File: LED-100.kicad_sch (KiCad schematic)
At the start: 101 parts, among them J2 LDA100_2_J2, J3 LDA100_2_J3, J4 LDA100_2_J4, J5 xtra, J7 Conn_01x01, J8 Conn_01x08, SW1 SW_SPDT, SW2 SW_SPST, U1 TLC5947DAP, U2 TLC5947DAP, U3 TLC5947DAP, U4 TEENSY 4.0

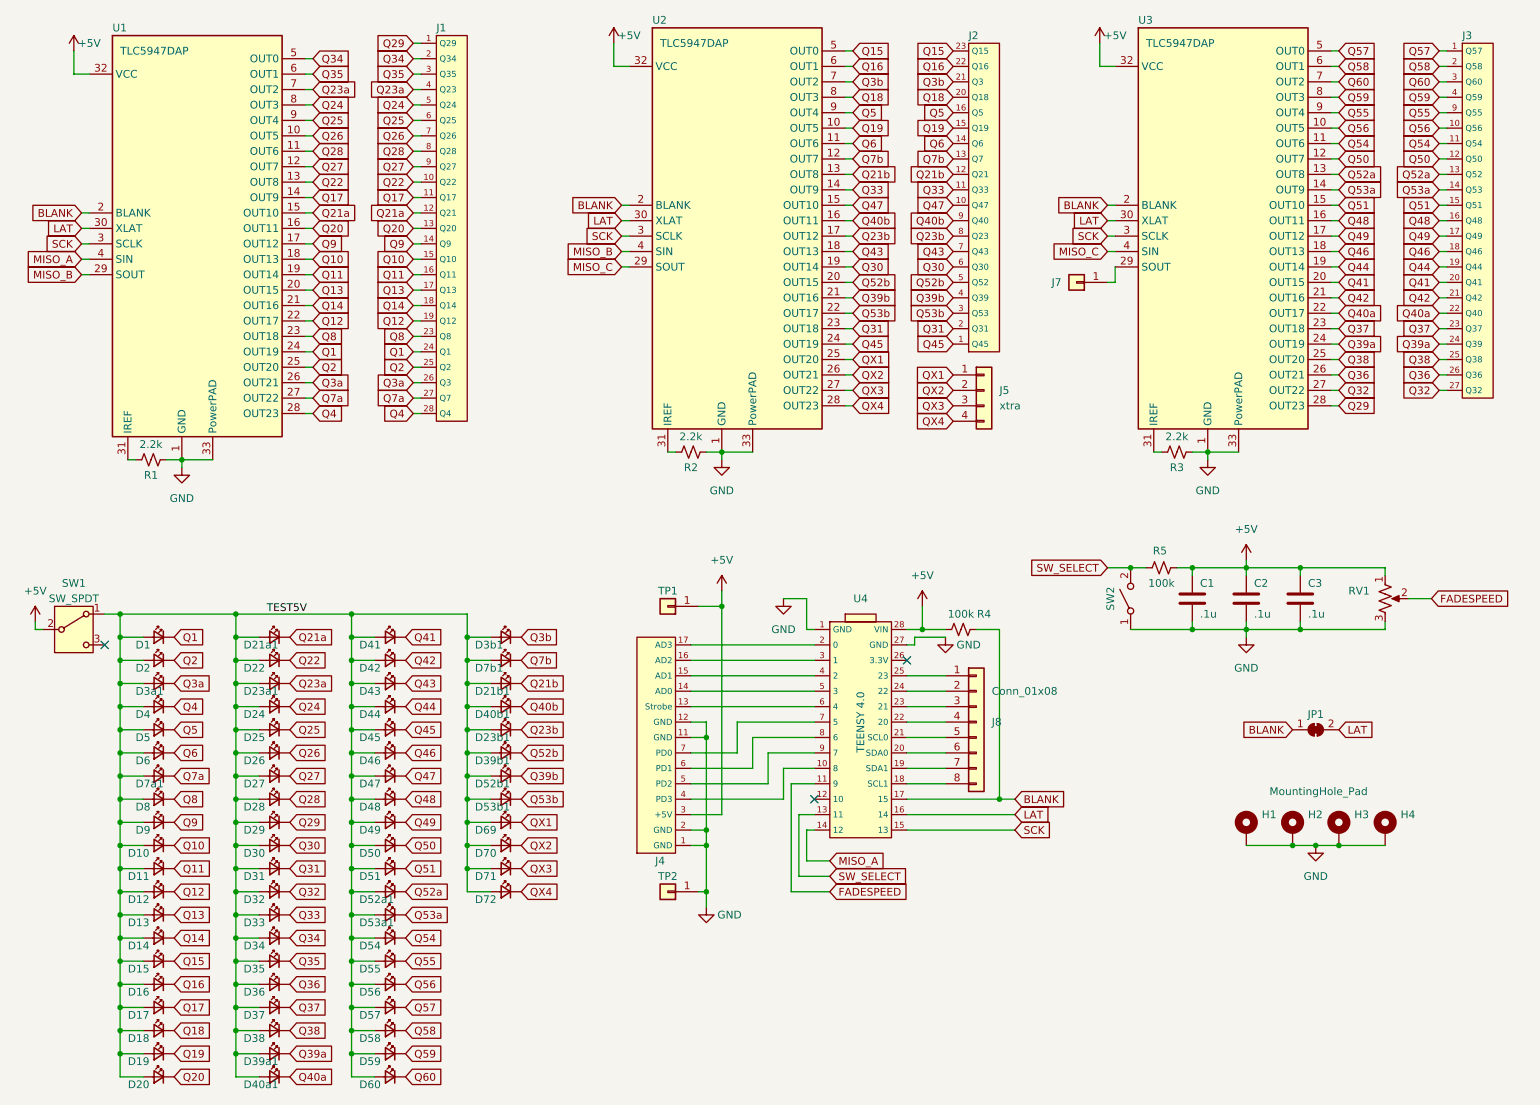
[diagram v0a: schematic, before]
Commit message: WIP
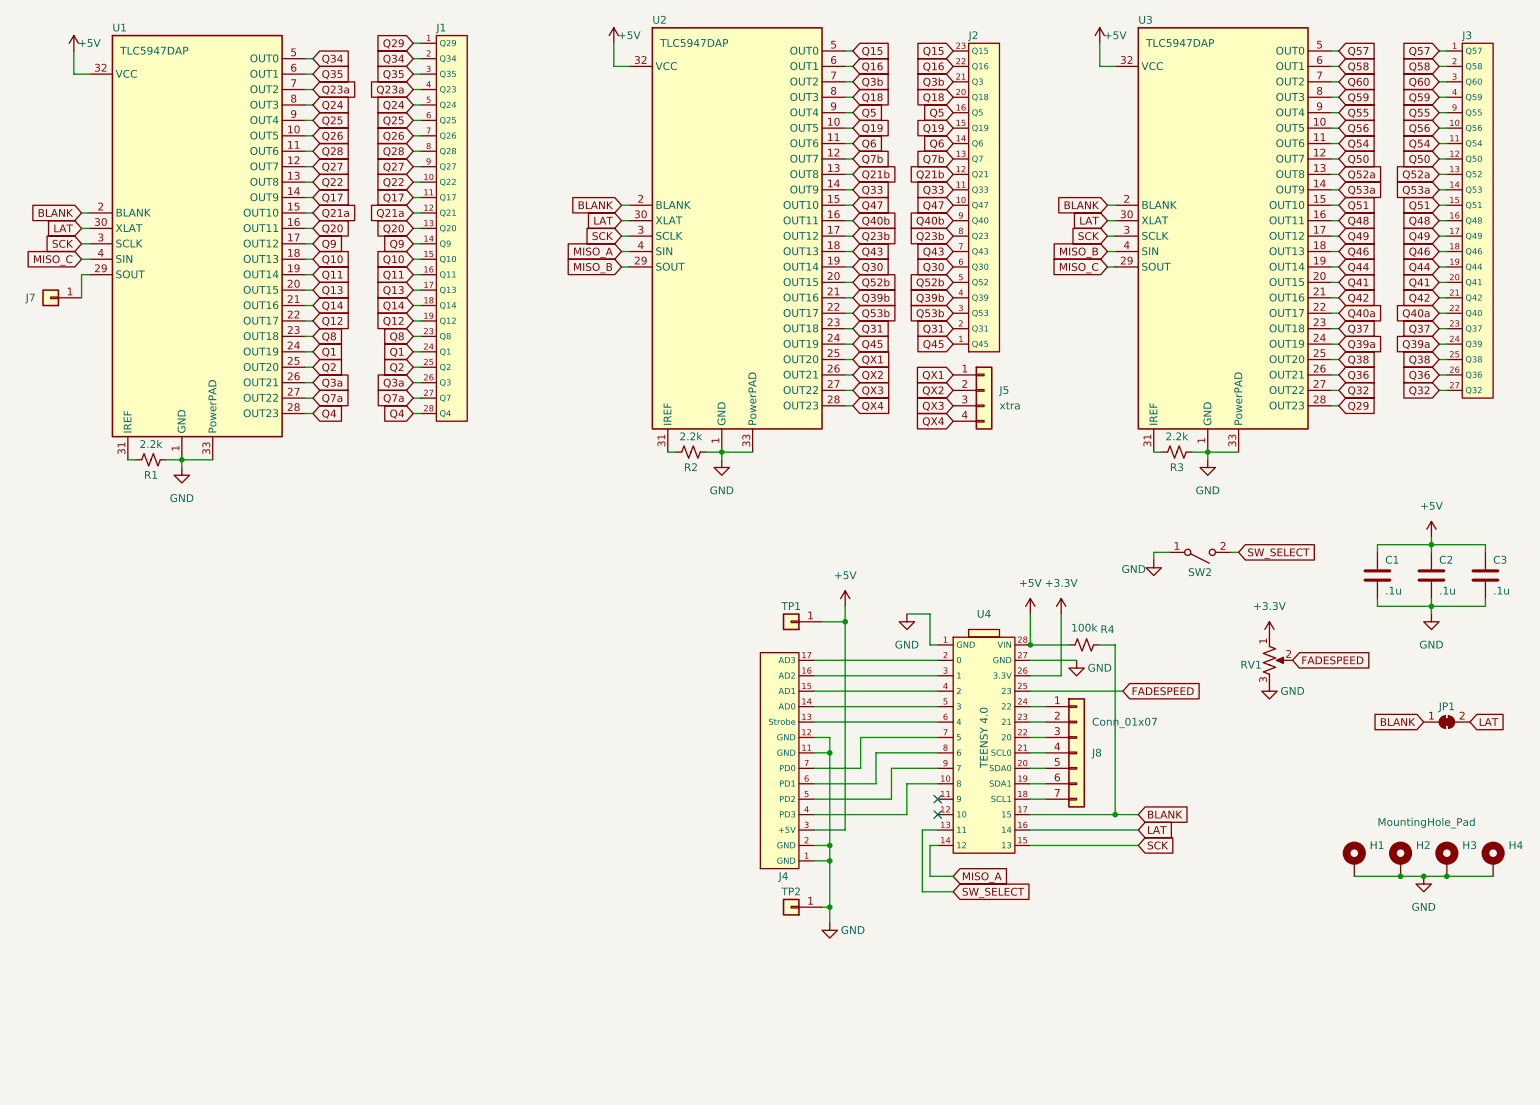
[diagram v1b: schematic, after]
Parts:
- removed D1, D10, D11, D12, D13, D14, D15, D16, D17, D18, D19, D2, D20, D21a1, D21b1, D22, D23a1, D23b1, D24, D25, D26, D27, D28, D29, D30, D31, D32, D33, D34, D35, D36, D37, D38, D39a1, D39b1, D3a1, D3b1, D4, D40a1, D40b1, D41, D42, D43, D44, D45, D46, D47, D48, D49, D5, D50, D51, D52a1, D52b1, D53a1, D53b1, D54, D55, D56, D57, D58, D59, D6, D60, D69, D70, D71, D72, D7a1, D7b1, D8, D9: LED_Small, LED_SMD:LED_0805_2012Metric_Pad1.15x1.40mm_HandSolder, symbol Device:LED_Small
- removed R5: 100k, Resistor_THT:R_Axial_DIN0204_L3.6mm_D1.6mm_P5.08mm_Horizontal, symbol Device:R_Small_US
- removed SW1: SW_SPDT, MyParts:SWITCH_SPDT-SLW-12689-4A-N-D, symbol Switch:SW_SPDT
- J8: value Conn_01x08 -> Conn_01x07; footprint Connector_PinHeader_2.54mm:PinHeader_1x08_P2.54mm_Vertical -> Connector_PinHeader_2.54mm:PinHeader_1x07_P2.54mm_Vertical; symbol Connector_Generic:Conn_01x08 -> Connector_Generic:Conn_01x07
- RV1: value R_Potentiometer_US -> 100k
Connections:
- net +5V: no longer RV1.1
- net FADESPEED: now also U4.25 (23); no longer U4.11 (9)
- net MISO_A: now also U2.4 (SIN); no longer U1.4 (SIN)
- net MISO_B: now also U2.29 (SOUT), U3.4 (SIN); no longer U1.29 (SOUT), U2.4 (SIN)
- net MISO_C: now also U1.4 (SIN), U3.29 (SOUT); no longer U2.29 (SOUT), U3.4 (SIN)
- net at U4.18 (SCL1): now also J8.7 (Pin_7); no longer J8.8 (Pin_8)
- net at U4.19 (SDA1): now also J8.6 (Pin_6); no longer J8.7 (Pin_7)
- net at U4.20 (SDA0): now also J8.5 (Pin_5); no longer J8.6 (Pin_6)
- net at U4.21 (SCL0): now also J8.4 (Pin_4); no longer J8.5 (Pin_5)
- net at U4.22 (20): now also J8.3 (Pin_3); no longer J8.4 (Pin_4)
- net at U4.23 (21): now also J8.2 (Pin_2); no longer J8.3 (Pin_3)
- net at U4.24 (22): now also J8.1 (Pin_1); no longer J8.2 (Pin_2)
- net +3.3V: now reaches U4.26 (3.3V)
- net +3.3V: now also RV1.1
- net at J7.1 (Pin_1): now also U1.29 (SOUT); no longer U3.29 (SOUT)
- no-connect marks 3 -> 2
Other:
- moved on the sheet: C1, C2, C3, H1, H2, H3, H4, J4, JP1, R4, RV1, SW2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
